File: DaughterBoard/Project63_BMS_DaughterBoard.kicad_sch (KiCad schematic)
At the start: 0 parts

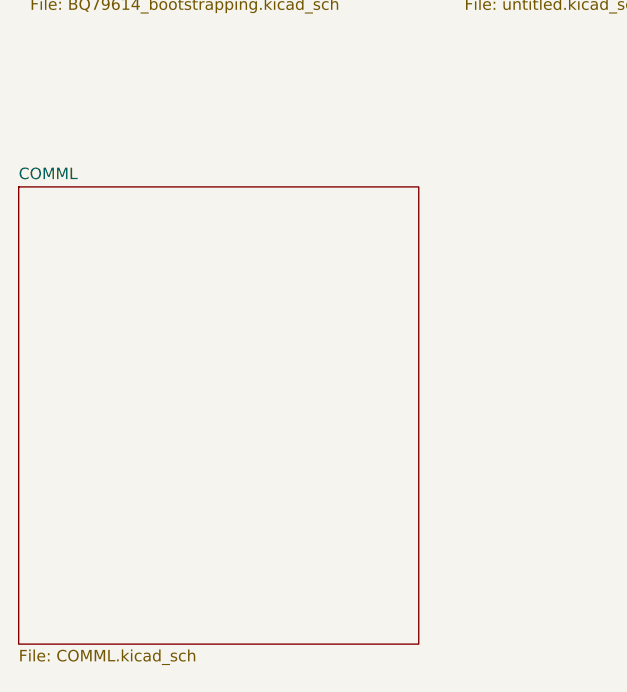
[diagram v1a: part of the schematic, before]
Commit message: Updates
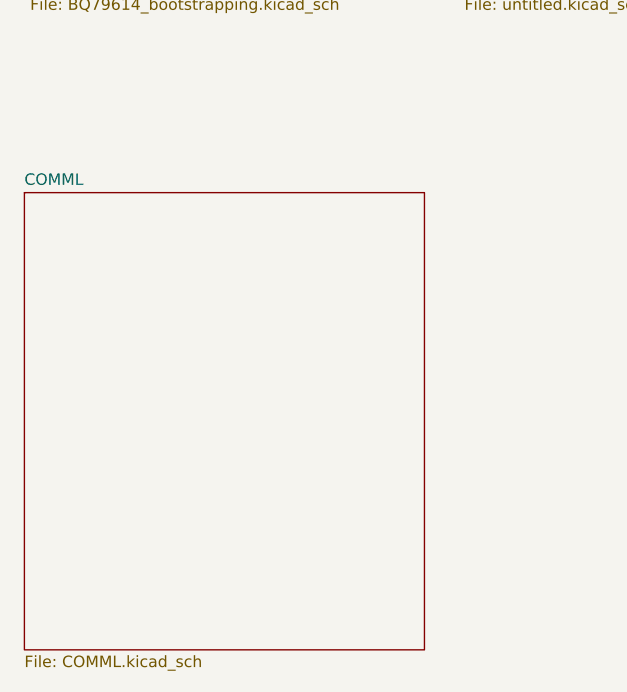
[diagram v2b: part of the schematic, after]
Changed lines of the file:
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@@
 	)
 	(sheet
-		(at 24.13 90.17)
+		(at 24.765 90.805)
 		(size 44.45 50.8)
 		(fields_autoplaced yes)
@@
 		)
 		(property "Sheetname" "COMML"
-			(at 24.13 89.4584 0)
+			(at 24.765 90.0934 0)
 			(effects
 				(font
@@
 		)
 		(property "Sheetfile" "COMML.kicad_sch"
-			(at 24.13 141.5546 0)
+			(at 24.765 142.1896 0)
 			(effects
 				(font
